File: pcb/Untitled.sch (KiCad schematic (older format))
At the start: 13 parts

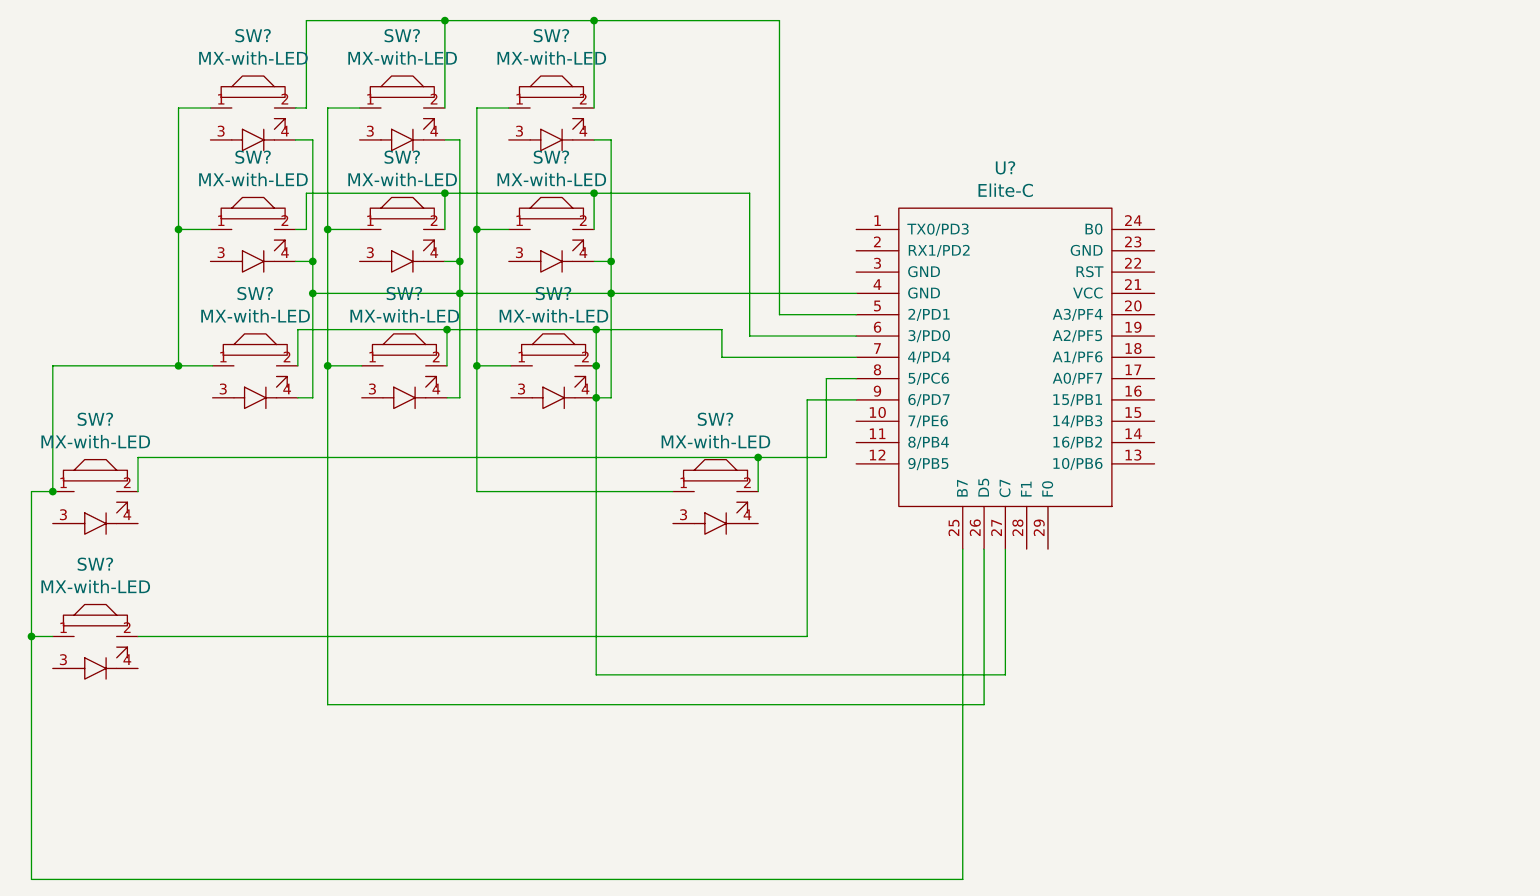
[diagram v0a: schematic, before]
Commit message: updated firmware and pcb schematics
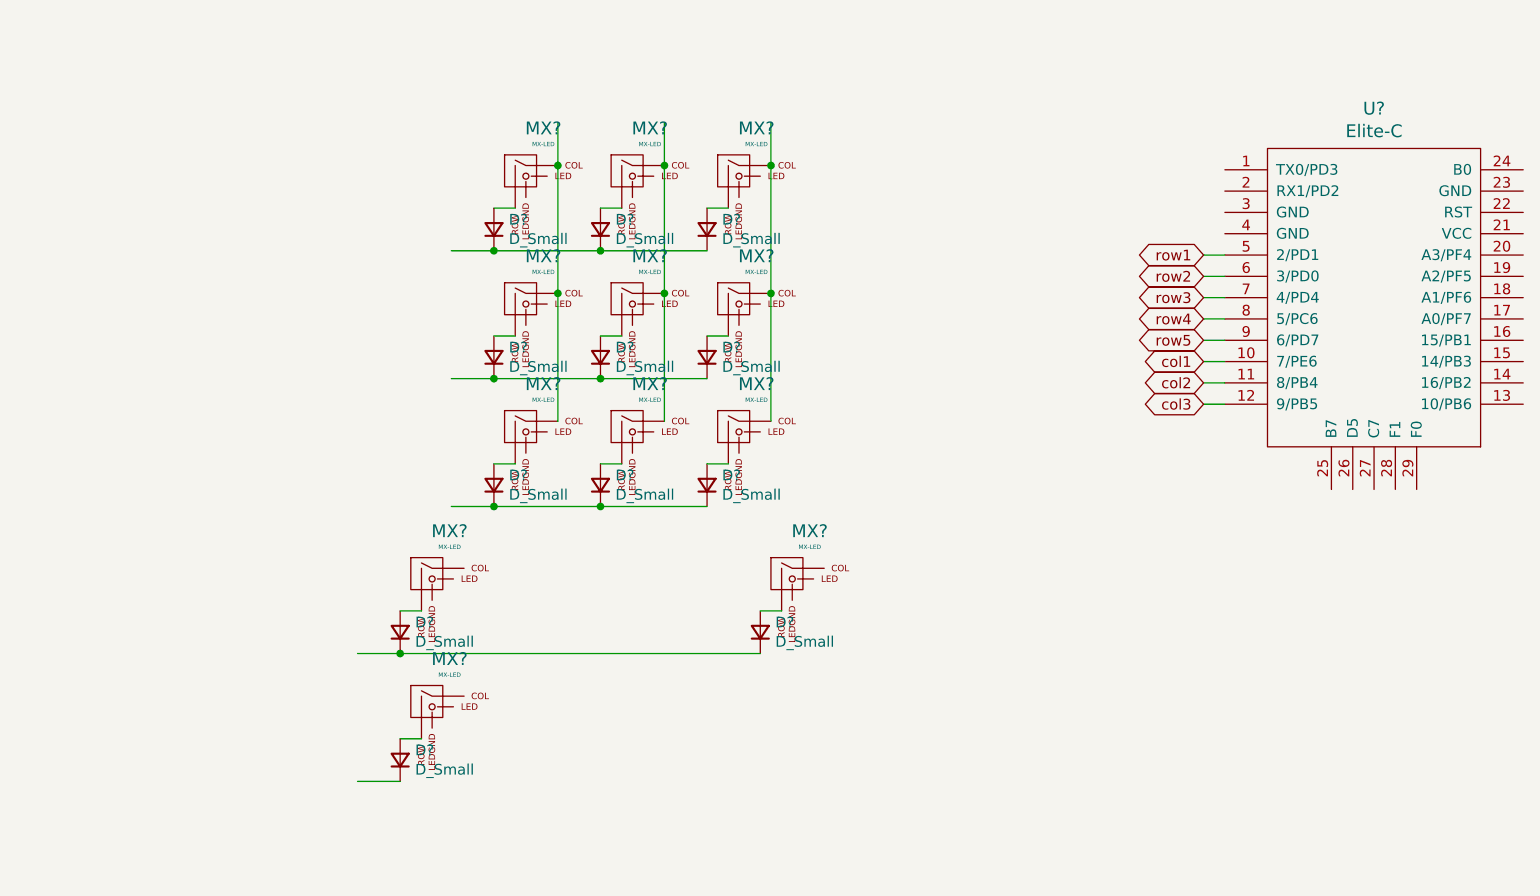
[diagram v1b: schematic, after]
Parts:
- removed SW? (x12): MX-with-LED, symbol keebio:MX-with-LED
- removed U?: Elite-C, symbol keebio:Elite-C
- added D? (x12): D_Small, symbol Device:D_Small
- added MX? (x12): MX-LED, symbol MX_Alps_Hybrid:MX-LED
- added U?: Elite-C, symbol keebio:Elite-C
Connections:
- net labels added: col1, col2, col3, row1, row2, row3, row4, row5
- wire segments 88 -> 41
